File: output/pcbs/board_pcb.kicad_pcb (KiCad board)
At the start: 2 copper layers, 138.7 x 126.5 mm, 62 parts

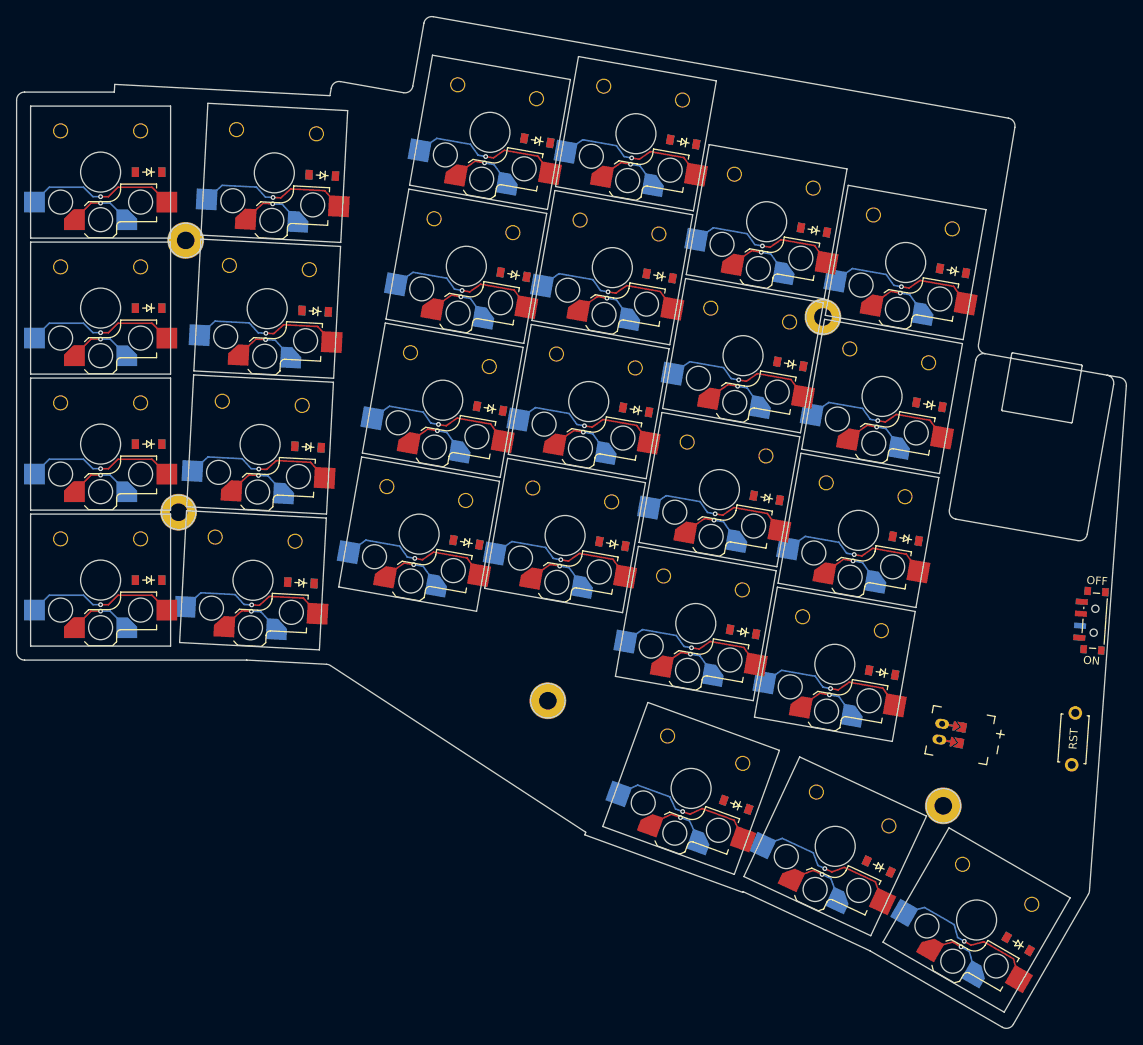
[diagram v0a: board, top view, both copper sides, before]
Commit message: Use irreversible config for easier design
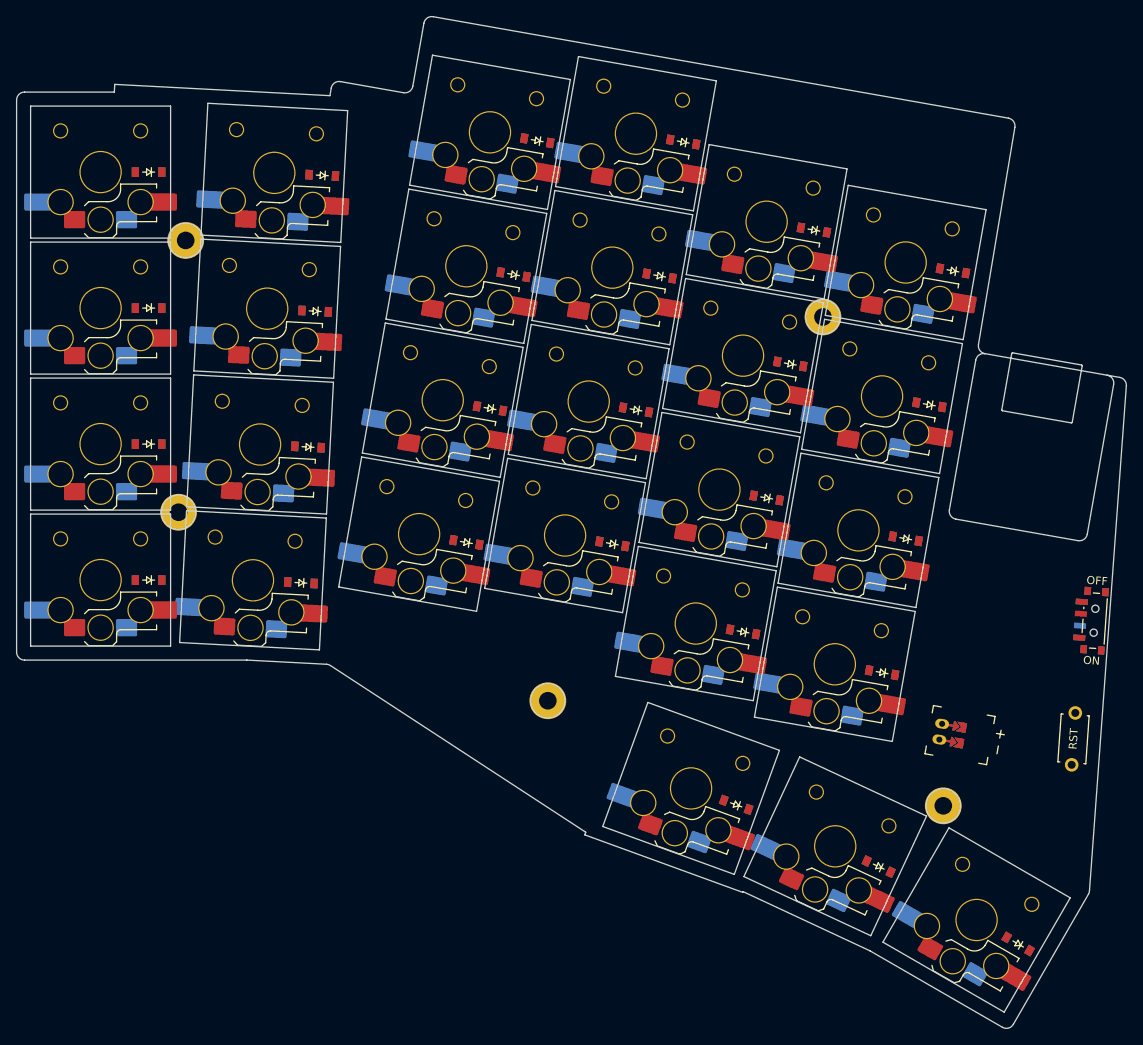
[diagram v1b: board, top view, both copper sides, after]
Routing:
- net col4: track 95.3 -> 0.00 mm, vias 5 -> 0
- net col3: track 95.3 -> 0.00 mm, vias 5 -> 0
- net col5: track 95.3 -> 0.00 mm, vias 5 -> 0
- net col1: track 76.3 -> 0.00 mm, vias 4 -> 0
- net col0: track 76.3 -> 0.00 mm, vias 4 -> 0
- net col2: track 76.3 -> 0.00 mm, vias 4 -> 0
- net far_thumb: track 8.27 -> 0.00 mm, vias 1 -> 0
- net near_thumb: track 8.27 -> 0.00 mm, vias 1 -> 0
- net pinky_home: track 8.27 -> 0.00 mm, vias 1 -> 0
- net pinky_bottom: track 8.27 -> 0.00 mm, vias 1 -> 0
- net pinky_upper: track 8.27 -> 0.00 mm, vias 1 -> 0
- net pinky_top: track 8.27 -> 0.00 mm, vias 1 -> 0
- net extra_pinky_upper: track 8.27 -> 0.00 mm, vias 1 -> 0
- net extra_pinky_top: track 8.27 -> 0.00 mm, vias 1 -> 0
- net extra_pinky_home: track 8.27 -> 0.00 mm, vias 1 -> 0
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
